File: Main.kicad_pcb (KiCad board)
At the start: 2 copper layers, 83.5 x 82.8 mm, 32 parts, among them J1 Conn_01x02, J2 Conn_01x02, J3 Conn_01x06, J4 Conn_01x02, J5 Conn_01x02, J6 Conn_01x03, J7 Conn_01x04, U1 DEV-16771, U2 K230D, U3 SeeeduinoXIAO, U4 AP63201WU, U6 AP63201WU

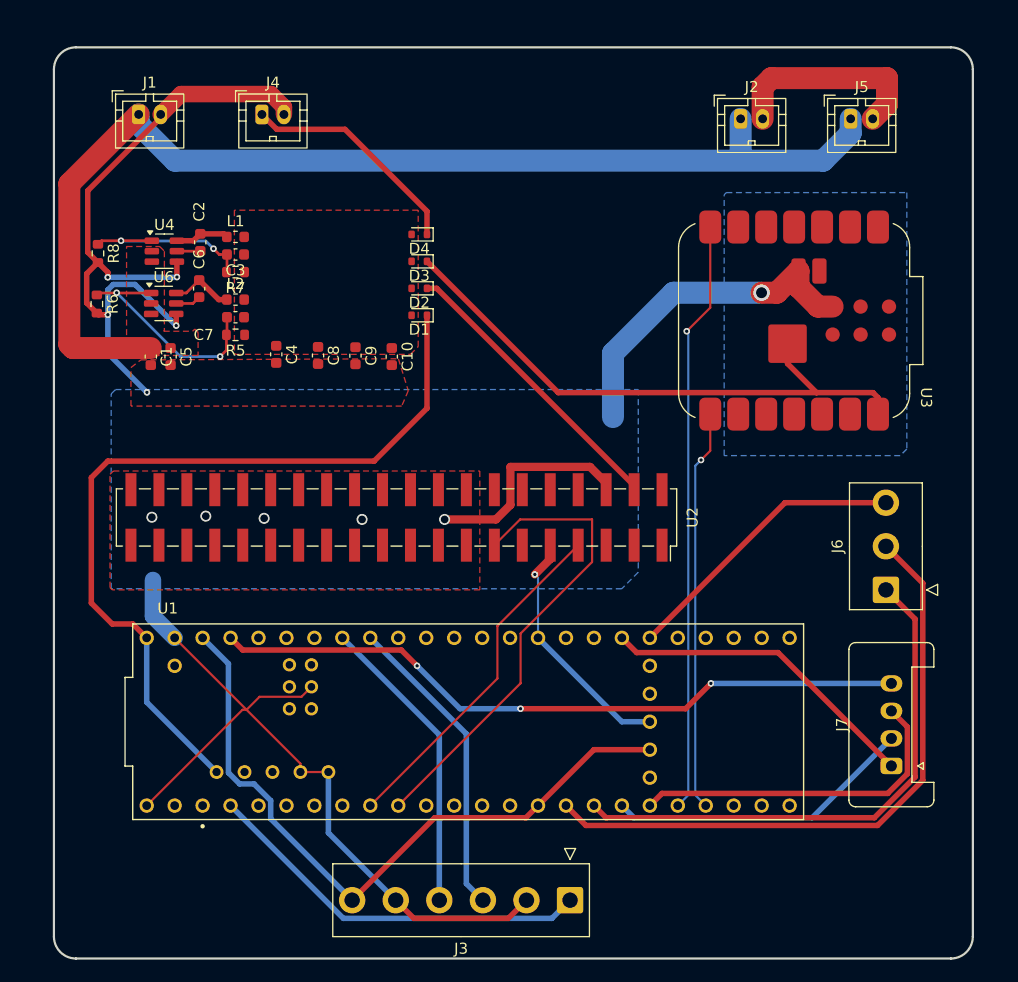
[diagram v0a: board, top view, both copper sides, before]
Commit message: Add files via upload
Done, forgive the trace lengths or I die
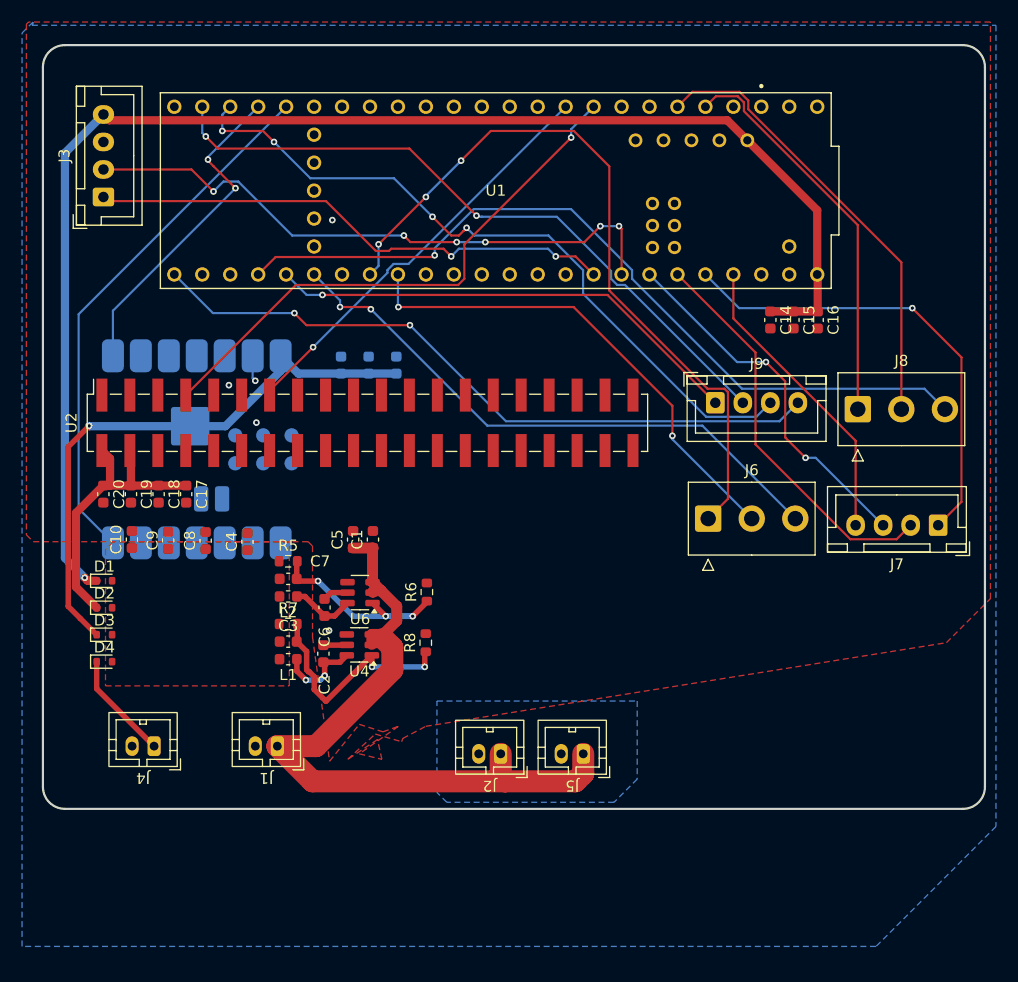
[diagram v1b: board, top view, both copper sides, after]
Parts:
- added C11: 0.1uF, Capacitor_SMD:C_0603_1608Metric, B.Cu at (99.6, 97.1)
- added C12: 22uF, Capacitor_SMD:C_0603_1608Metric, B.Cu at (97.1, 97.1)
- added C13: 1uF, Capacitor_SMD:C_0603_1608Metric, B.Cu at (94.6, 97.1)
- added C14: 22uF, Capacitor_SMD:C_0603_1608Metric, F.Cu at (133.6, 93.0)
- added C15: 1uF, Capacitor_SMD:C_0603_1608Metric, F.Cu at (135.7, 93.0)
- added C16: 0.1uF, Capacitor_SMD:C_0603_1608Metric, F.Cu at (137.9, 93.0)
- added C17: 0.1uF, Capacitor_SMD:C_0603_1608Metric, F.Cu at (80.5, 108.8)
- added C18: 22uF, Capacitor_SMD:C_0603_1608Metric, F.Cu at (78.0, 108.8)
- added C19: 1uF, Capacitor_SMD:C_0603_1608Metric, F.Cu at (75.5, 108.8)
- added C20: 47uF, Capacitor_SMD:C_0603_1608Metric, F.Cu at (73.0, 108.8)
- added J8: Conn_01x03, Connector_TE-Connectivity:TE_826576-3_1x03_P3.96mm_Vertical, F.Cu at (141.5, 101.1)
- added J9: Conn_01x04, Connector_JST:JST_XH_B4B-XH-A_1x04_P2.50mm_Vertical, F.Cu at (128.6, 100.5)
- J3: value Conn_01x06 -> Conn_01x04; footprint Connector_TE-Connectivity:TE_826576-6_1x06_P3.96mm_Vertical -> Connector_JST:JST_XH_B4B-XH-A_1x04_P2.50mm_Vertical
- J7: footprint Connector_Stocko:Stocko_MKS_1654-6-0-404_1x4_P2.50mm_Vertical -> Connector_JST:JST_XH_B4B-XH-A_1x04_P2.50mm_Vertical
- U3: moved to B.Cu
- moved J3 76.7 mm to (73.0, 81.8), turned to 90 degrees
- moved J5 62.6 mm to (116.6, 132.4), turned to 180 degrees
- moved J2 61.7 mm to (109.1, 132.4), turned to 180 degrees
- moved J1 58.8 mm to (88.8, 131.7), turned to 180 degrees
- moved J4 58.2 mm to (77.6, 131.7), turned to 180 degrees
- moved U3 55.5 mm to (81.5, 104.7), turned to 90 degrees
- moved U1 48.3 mm to (108.7, 81.2), turned to 180 degrees
- moved D4 48.2 mm to (73.1, 124.0), turned to 0 degrees
- moved R8 46.2 mm to (102.3, 122.3), turned to 90 degrees
- moved D3 44.4 mm to (73.1, 121.6), turned to 0 degrees
- moved D2 40.8 mm to (73.1, 119.1), turned to 0 degrees
- moved U4 39.9 mm to (96.2, 122.5), turned to 180 degrees
- moved R6 39.8 mm to (102.4, 117.7), turned to 90 degrees
- moved C2 39.0 mm to (93.0, 123.3), turned to -90 degrees
- moved L1 38.7 mm to (89.8, 123.8), turned to 180 degrees
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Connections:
- J3 pad 1: /INT -> /SDA
- J3 pad 2: GND -> /SCL
- J3 pad 3: /SDA -> GND
- J3 pad 4: /SCL -> Net-(D1-K)
- U1 pad 2: /INT -> unconnected-(U1-OUT2-Pad2)
- U1 pad 20: unconnected-(U1-A6-Pad20) -> /AIN1
- U1 pad 21: unconnected-(U1-A7-Pad21) -> /AIN2
- U1 pad 22: unconnected-(U1-A8-Pad22) -> /PWMA
- U1 pad 24: /BIN2 -> unconnected-(U1-A10-Pad24)
- U1 pad 25: /BIN1 -> unconnected-(U1-A11-Pad25)
- U1 pad 26: /AIN2 -> unconnected-(U1-A12-Pad26)
- U1 pad 27: /AIN1 -> unconnected-(U1-A13-Pad27)
- U1 pad 3: unconnected-(U1-LRCLK2-Pad3) -> /BIN1_1
- U1 pad 3.3V_1: +3.3V -> Net-(U1-3.3V-Pad3.3V_1)
- U1 pad 3.3V_2: +3.3V -> Net-(U1-3.3V-Pad3.3V_1)
- U1 pad 3.3V_3: +3.3V -> Net-(U1-3.3V-Pad3.3V_1)
- U1 pad 30: unconnected-(U1-CRX3-Pad30) -> /AIN1_1
- U1 pad 31: unconnected-(U1-CTX3-Pad31) -> /AIN2_1
- U1 pad 33: unconnected-(U1-MCLK2-Pad33) -> /STBY_1
- U1 pad 36: unconnected-(U1-CS2-Pad36) -> /PWMB_1
- U1 pad 37: unconnected-(U1-CS3-Pad37) -> /PWMA_1
- U1 pad 39: /PWMA -> unconnected-(U1-A15-Pad39)
- U1 pad 4: unconnected-(U1-BCLK2-Pad4) -> /BIN2_1
- U1 pad 40: unconnected-(U1-A16-Pad40) -> /BIN1
- U1 pad 41: unconnected-(U1-A17-Pad41) -> /BIN2
- U1 pad VUSB: /VUSB -> unconnected-(U1-PadVUSB)
- U3 pad 13: unconnected-(U3-GND-Pad13) -> GND
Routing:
- net GND: track 211.4 -> 2.37 mm, vias 12 -> 5
- net /PWMB_1: track 0.00 -> 73.4 mm, vias 0 -> 1
- net /AIN1_1: track 0.00 -> 65.9 mm, vias 0 -> 4
- net /STBY_1: track 0.00 -> 63.2 mm, vias 0 -> 2
- net +3.3V: track 63.0 -> 0.00 mm
- net /AIN2_1: track 0.00 -> 62.2 mm, vias 0 -> 2
- net Net-(D1-K): track 74.1 -> 127.5 mm, vias 0 -> 1
- net /PWMA_1: track 0.00 -> 43.8 mm, vias 0 -> 1
- net /BIN2_1: track 0.00 -> 41.1 mm
- net +6.6V: track 103.2 -> 65.1 mm
- net /BIN1_1: track 0.00 -> 36.3 mm
- net /STBY: track 63.7 -> 27.4 mm, vias 3 -> 0
- net /INT: track 35.8 -> 0.00 mm
- net /SCL: track 27.5 -> 55.6 mm, vias 0 -> 6
- net /PWMB: track 26.5 -> 53.3 mm, vias 0 -> 2
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- added copper zone on B.Cu, net MGND
- removed copper zone on F.Cu, net +6.6V
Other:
- board size 83.5 x 82.8 mm -> 85.6 x 69.4 mm
